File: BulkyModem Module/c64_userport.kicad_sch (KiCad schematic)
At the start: 1 part, among them J5 C64_Modem_IDC

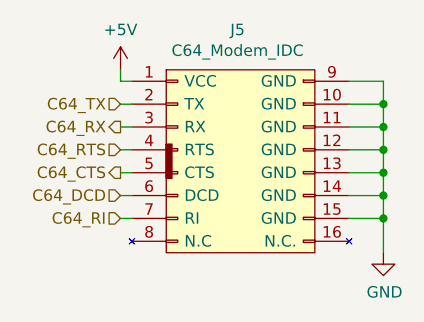
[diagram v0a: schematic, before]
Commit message: Exported files
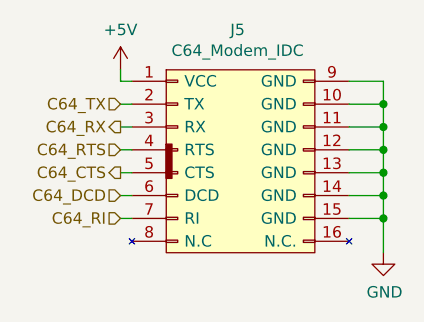
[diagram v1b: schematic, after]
